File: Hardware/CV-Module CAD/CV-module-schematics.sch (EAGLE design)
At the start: 12 parts, among them U1 AD5611BKSZ, U2 AD5611BKSZ, U3 AD5611BKSZ, U4 AD5611BKSZ, U5 AD5611BKSZ, U6 AD5611BKSZ, U7 AD5611BKSZ, U8 AD5611BKSZ

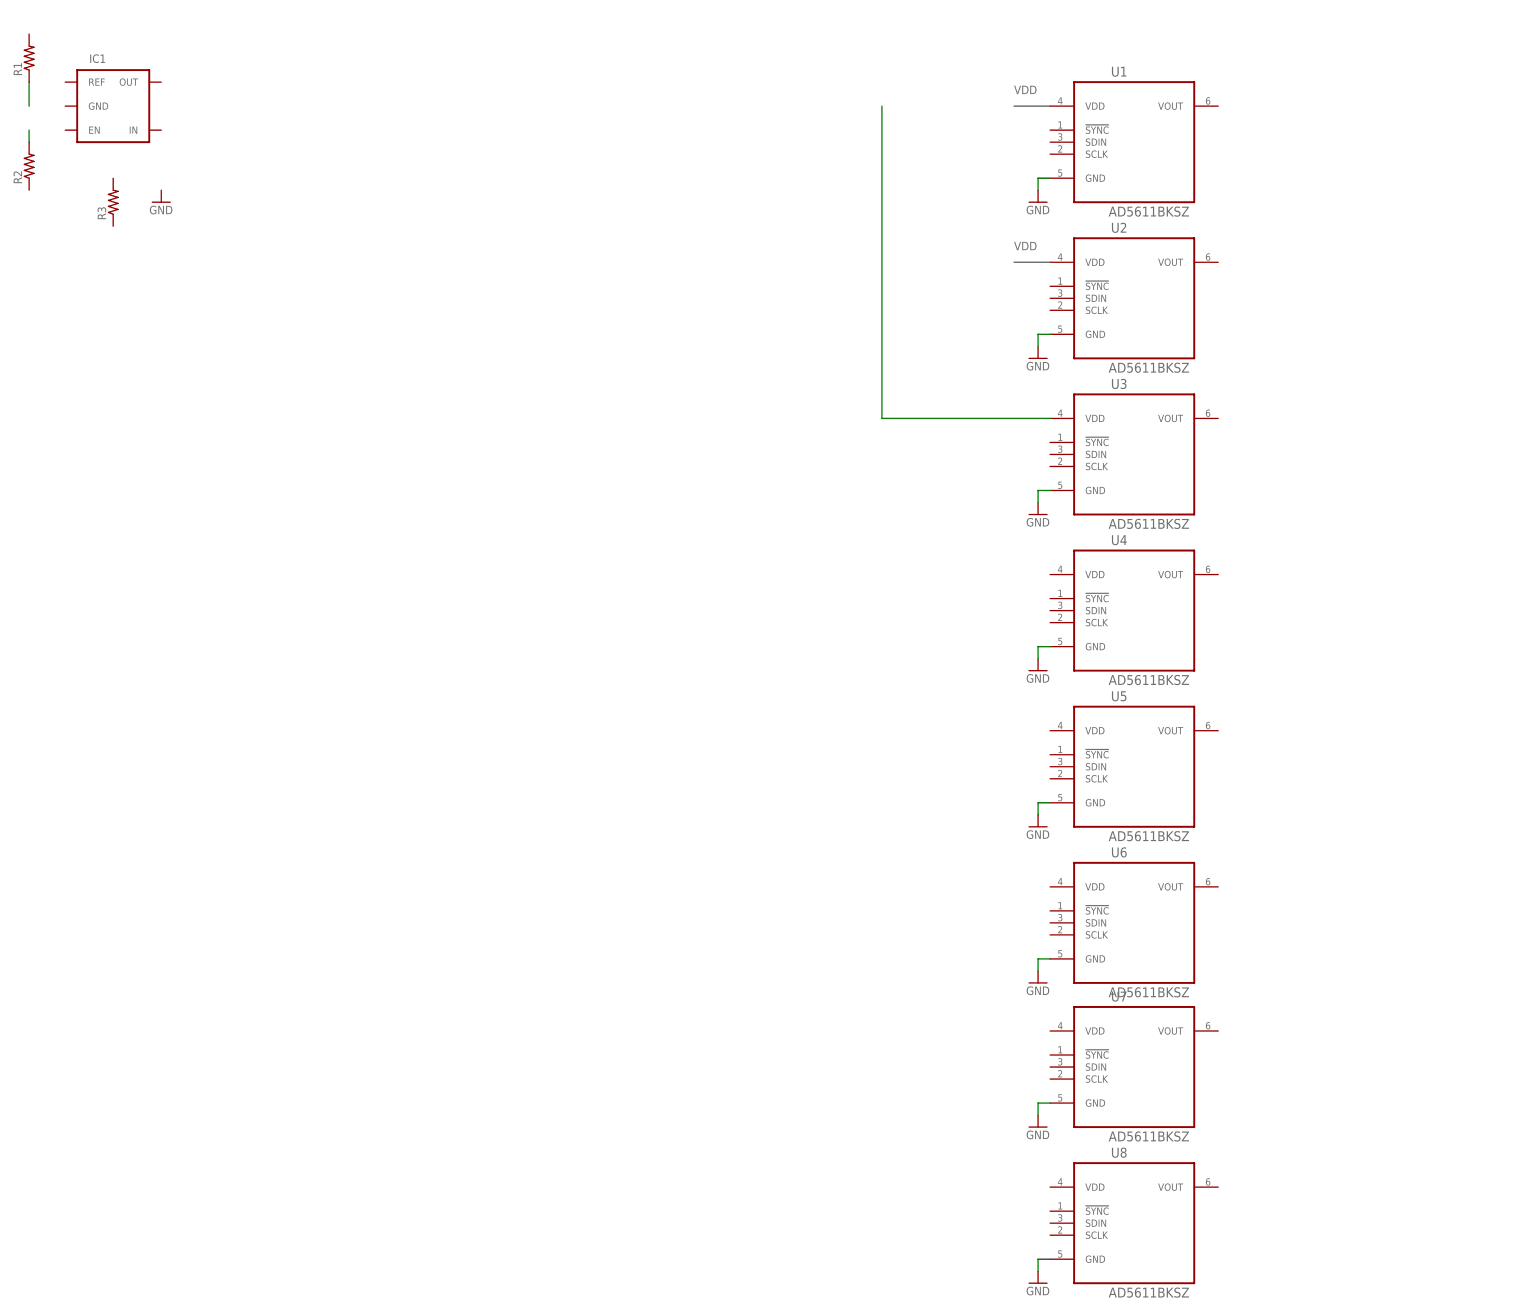
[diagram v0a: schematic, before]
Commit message: working on eagle-project
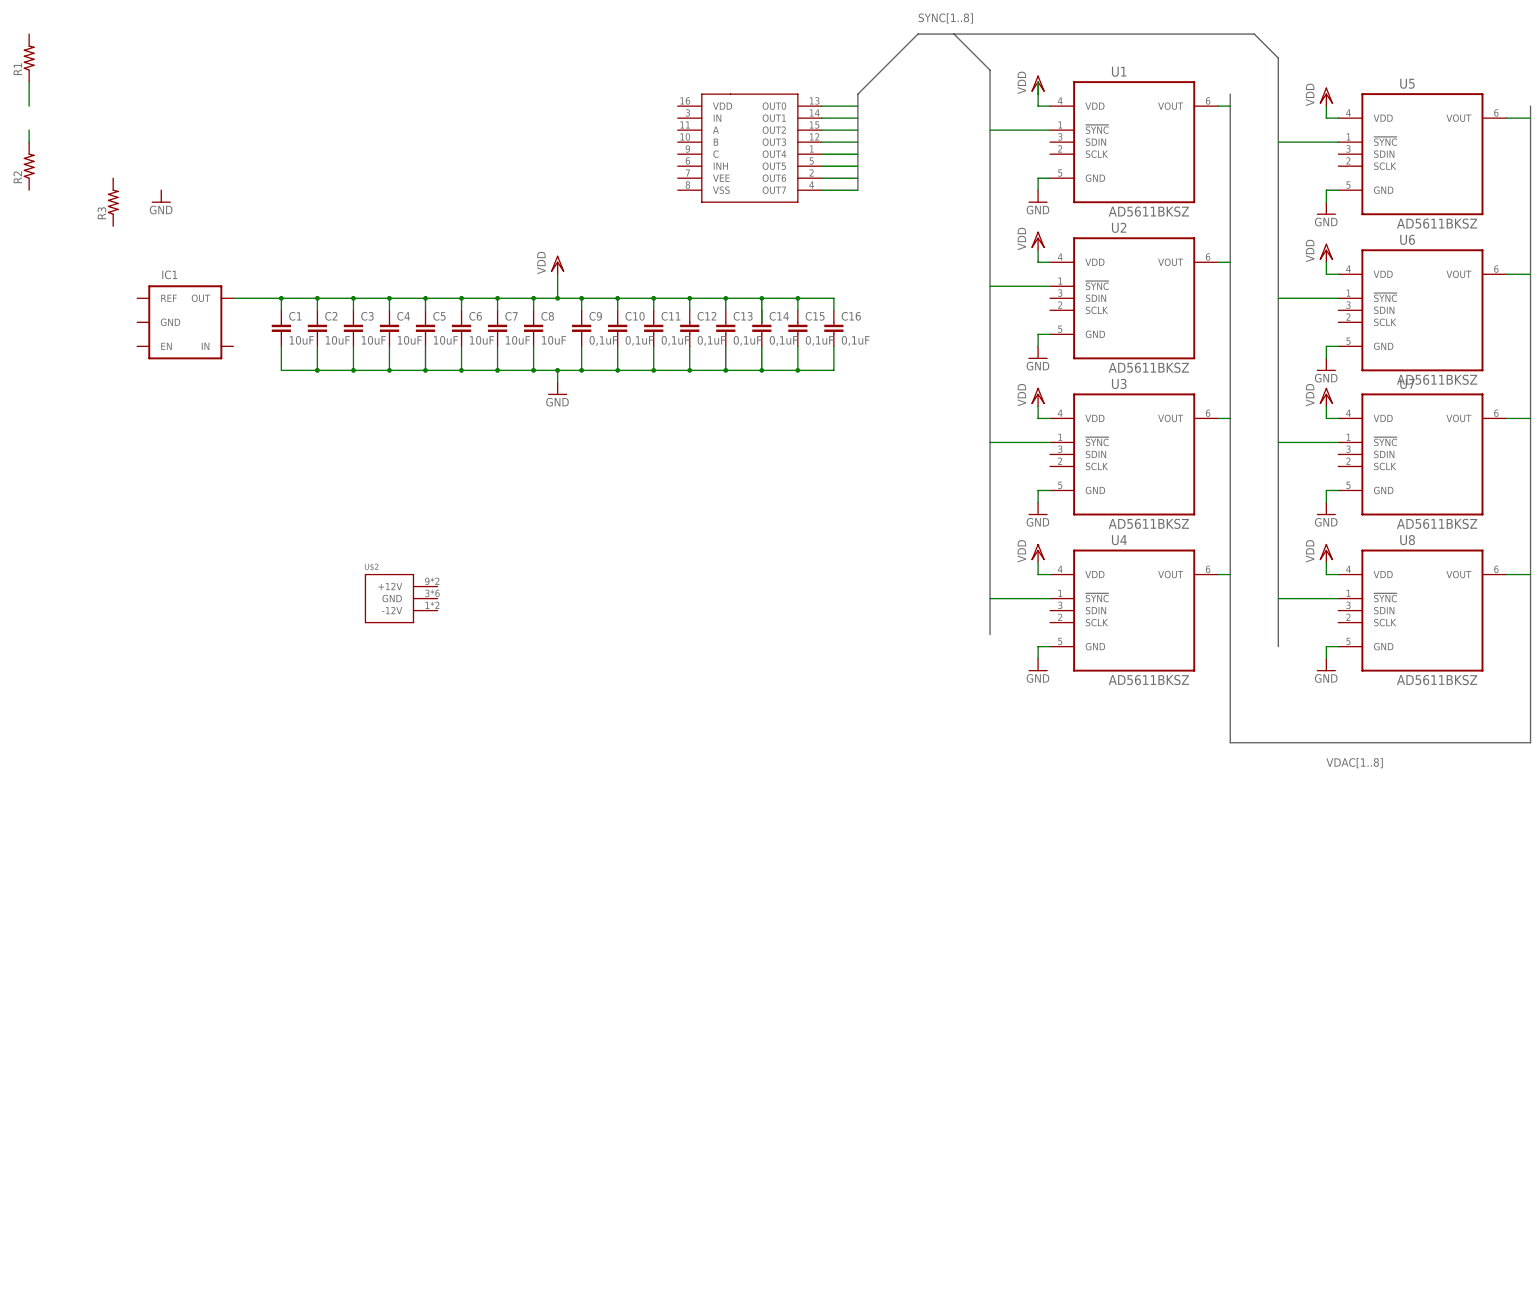
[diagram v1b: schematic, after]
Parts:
- added C1, C2, C3, C4, C5, C6, C7, C8: 10uF, resistor:C-EUC1206
- added C10, C11, C12, C13, C14, C15, C16, C9: 0,1uF, resistor:C-EUC0603
- added U$1: CD4051BM96, halo-electronics:CD4051BM96
- added U$2: POWER_SIMPLE10, eurorack:POWER_SIMPLE10
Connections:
- new net SYNC1: U$1.OUT0, U1.!SYNC
- new net SYNC2: U$1.OUT1, U2.!SYNC
- new net SYNC3: U$1.OUT2, U3.!SYNC
- new net SYNC4: U$1.OUT3, U4.!SYNC
- new net SYNC5: U$1.OUT4, U5.!SYNC
- new net SYNC6: U$1.OUT5, U6.!SYNC
- new net SYNC7: U$1.OUT6, U7.!SYNC
- new net SYNC8: U$1.OUT7, U8.!SYNC
- new net VDAC1: U1.VOUT
- new net VDAC2: U2.VOUT
- new net VDAC3: U3.VOUT
- new net VDAC4: U4.VOUT
- new net VDAC5: U5.VOUT
- new net VDAC6: U6.VOUT
- new net VDAC7: U7.VOUT
- new net VDAC8: U8.VOUT
- net GND: now also C1.2, C10.2, C11.2, C12.2, C13.2, C14.2, C15.2, C16.2, C2.2, C3.2, C4.2, C5.2, C6.2, C7.2, C8.2, C9.2
- net VDD: now also C1.1, C10.1, C11.1, C12.1, C13.1, C15.1, C16.1, C2.1, C3.1, C4.1, C5.1, C6.1, C7.1, C8.1, C9.1, IC1.OUT, U1.VDD, U2.VDD, U4.VDD, U5.VDD, U6.VDD, U7.VDD, U8.VDD
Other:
- moved on the sheet: IC1, U5, U6, U7, U8
